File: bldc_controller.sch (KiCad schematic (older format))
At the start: 147 parts, among them J1 Conn_01x06_Male, J2 Banana_Jack, J3 Banana_Jack, Q1 2N7002E, Q10 IRLB8721PBF, Q11 IRLB8721PBF, Q2 DMN65D8L-7, Q3 DMN65D8L-7, Q4 MMBT3904, Q5 IRF4905, Q6 IRLB8721PBF, Q7 IRLB8721PBF, Q8 IRLB8721PBF, Q9 IRLB8721PBF, SW1 1301.9314, SW2 D6C50 F1 LFS, SW3 D6C40 F1 LFS, U1 ATmega328P-PU, U10 IRS2004, U2 SN74LVC1G11DBVR, U3 uA7810, U4 LM7805_TO220, U5 CD4044BE, U6 LM339, U7 MCP601-xP, U8 IRS2004, U9 IRS2004, Y1 9B-16.000MBBK-B

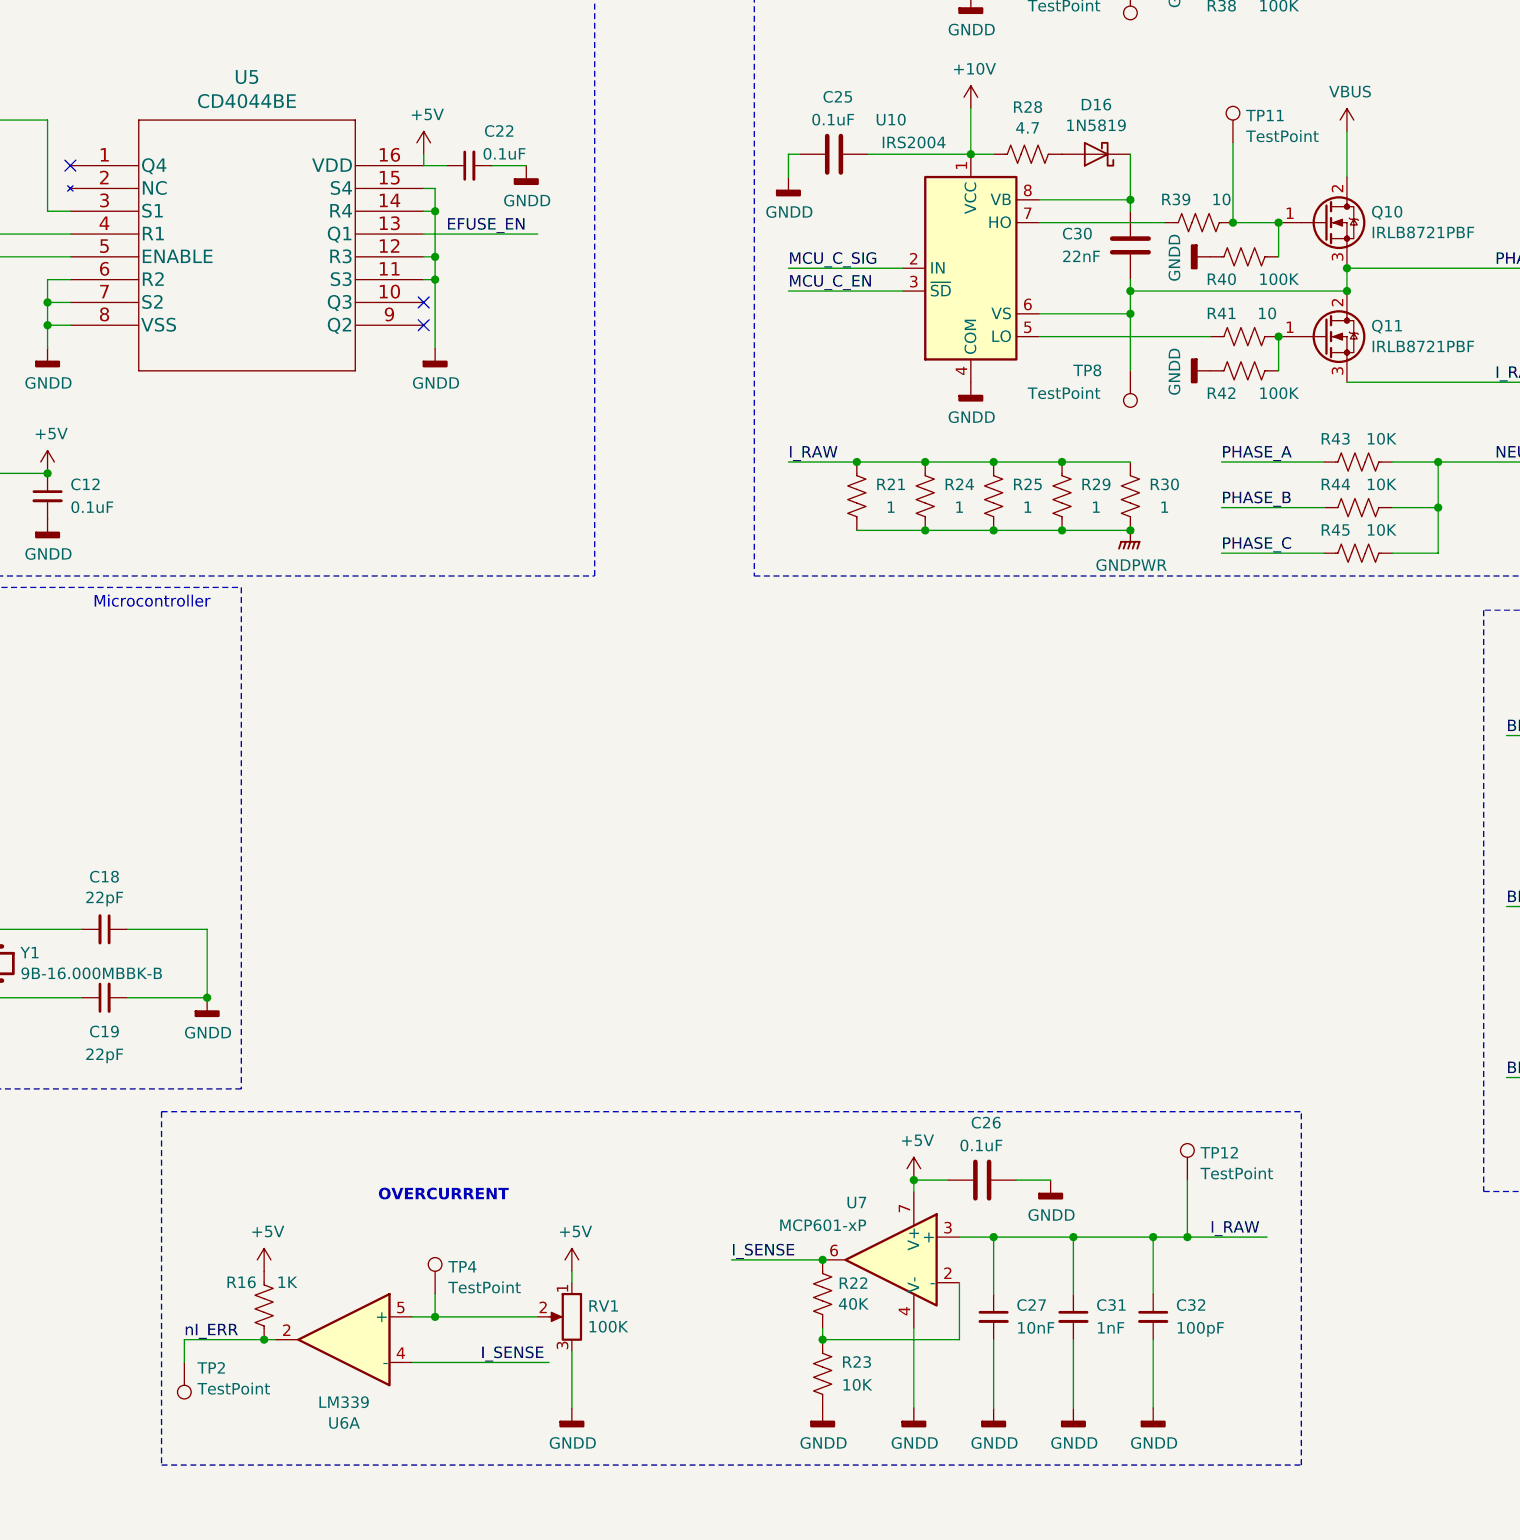
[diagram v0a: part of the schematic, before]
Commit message: Manual Revert
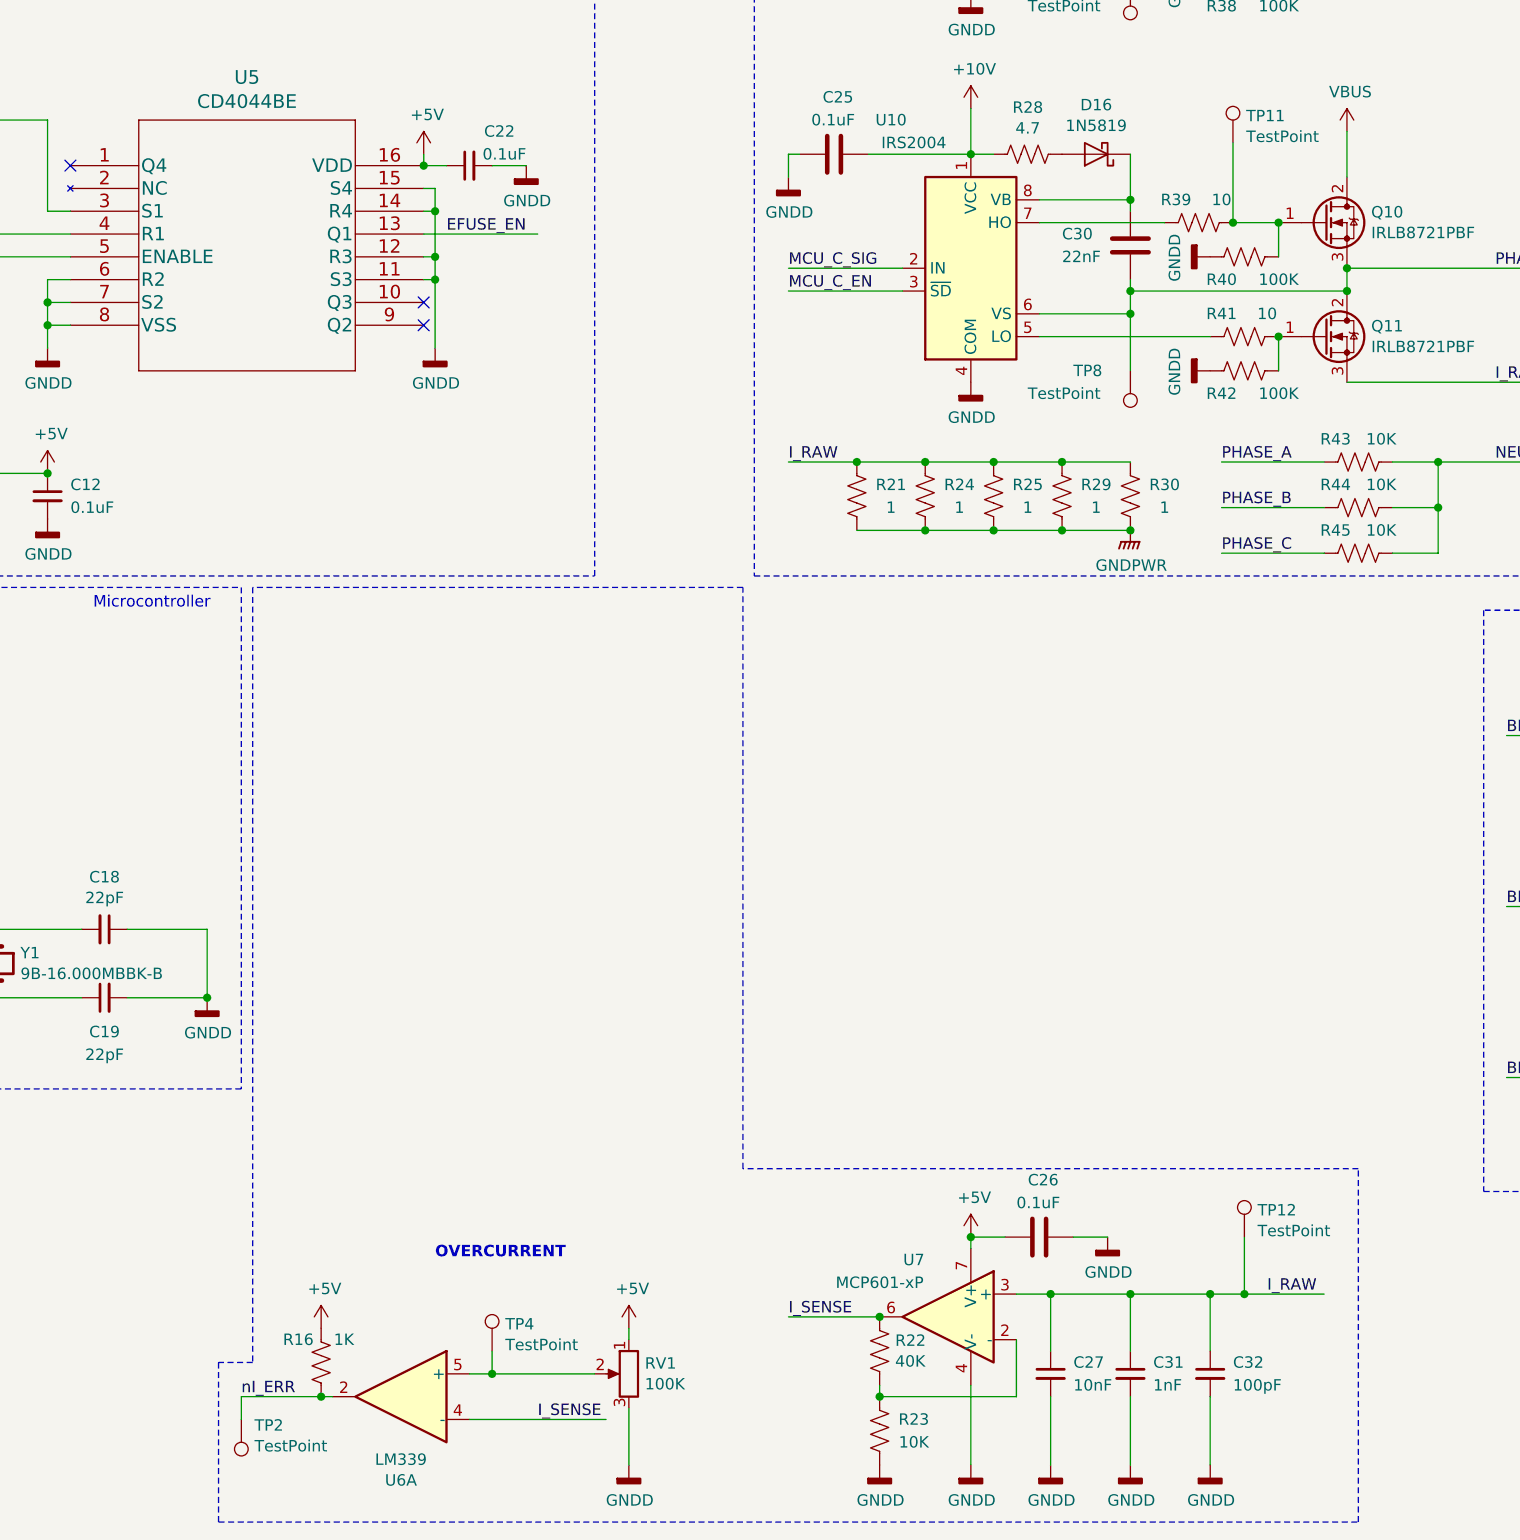
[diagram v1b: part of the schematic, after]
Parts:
- D10, D11: footprint Diode_THT:D_DO-35_SOD27_P7.62mm_Horizontal -> Diode_SMD:D_SOD-323_HandSoldering
- D14, D15, D16: footprint Diode_THT:D_DO-41_SOD81_P10.16mm_Horizontal -> Diode_SMD:D_SOD-123
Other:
- moved on the sheet: C26, C27, C31, C32, R16, R22, R23, RV1, TP12, TP2, TP4, U6A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
